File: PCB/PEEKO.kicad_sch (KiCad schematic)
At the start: 26 parts, among them J1 Rasberry PI Pico, J2 Conn_02x15_Odd_Even, J3 Conn_01x02_Pin, J4 Conn_01x02_Pin, U1 TXU0104, U2 TXU0104, U3 TXU0104, U4 TXU0104, U5 TXU0104, U6 TXU0104

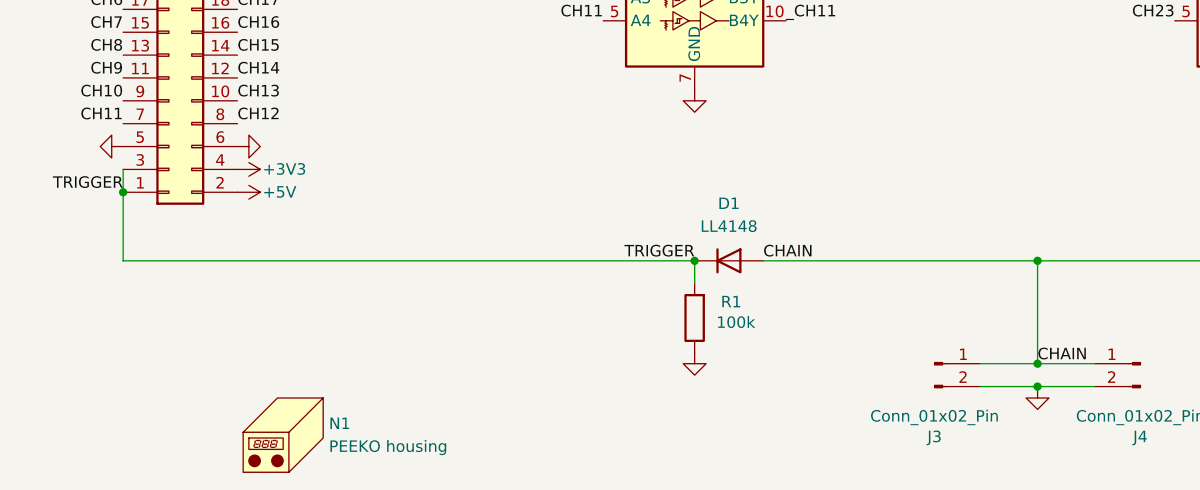
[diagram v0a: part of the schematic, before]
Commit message: boms
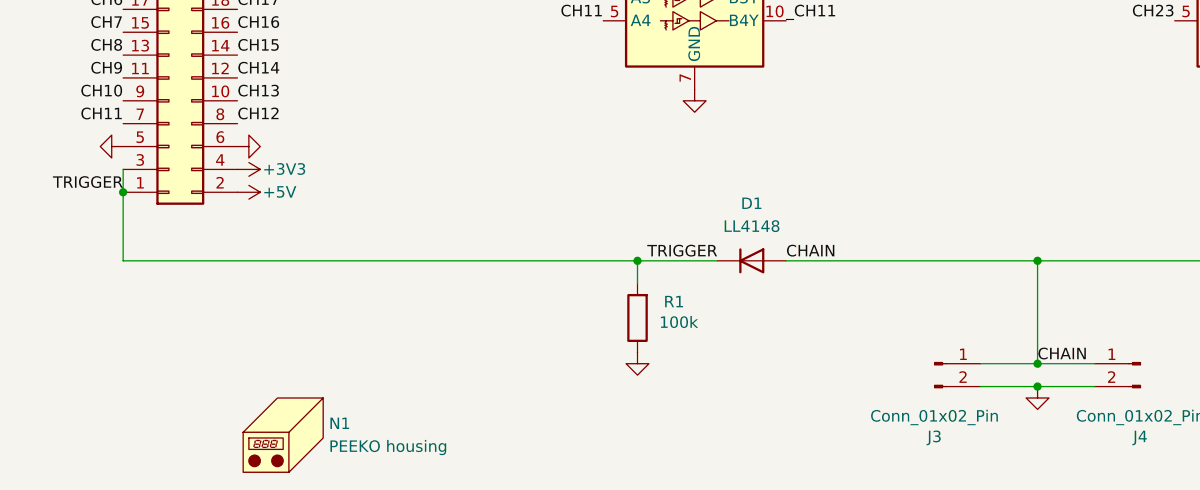
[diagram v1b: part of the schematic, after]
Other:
- moved on the sheet: D1, R1
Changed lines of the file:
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@@
 	)
 	(junction
-		(at 95.25 158.75)
-		(diameter 0)
-		(color 0 0 0 0)
-	)
-	(junction
 		(at 53.34 57.15)
 		(diameter 0)
@@
 	)
 	(junction
+		(at 88.9 158.75)
+		(diameter 0)
+		(color 0 0 0 0)
+	)
+	(junction
 		(at 266.7 101.6)
 		(diameter 0)
@@
 	(wire
 		(pts
-			(xy 95.25 158.75) (xy 95.25 161.29)
+			(xy 223.52 71.12) (xy 223.52 73.66)
 		)
 		(stroke
@@
 	(wire
 		(pts
-			(xy 223.52 71.12) (xy 223.52 73.66)
+			(xy 22.86 41.91) (xy 22.86 44.45)
 		)
 		(stroke
@@
 	(wire
 		(pts
-			(xy 22.86 41.91) (xy 22.86 44.45)
+			(xy 22.86 76.2) (xy 26.67 76.2)
 		)
 		(stroke
@@
 	(wire
 		(pts
-			(xy 22.86 76.2) (xy 26.67 76.2)
+			(xy 22.86 69.85) (xy 22.86 76.2)
 		)
 		(stroke
@@
 	(wire
 		(pts
-			(xy 22.86 69.85) (xy 22.86 76.2)
+			(xy 88.9 158.75) (xy 97.79 158.75)
 		)
 		(stroke
@@
 	(wire
 		(pts
+			(xy 88.9 158.75) (xy 88.9 161.29)
+		)
+		(stroke
+			(width 0)
+			(type default)
+		)
+	)
+	(wire
+		(pts
 			(xy 215.9 121.92) (xy 215.9 114.3)
 		)
@@
 	(wire
 		(pts
-			(xy 102.87 158.75) (xy 133.35 158.75)
+			(xy 105.41 158.75) (xy 133.35 158.75)
 		)
 		(stroke
@@
 	(wire
 		(pts
-			(xy 31.75 158.75) (xy 95.25 158.75)
+			(xy 31.75 158.75) (xy 88.9 158.75)
 		)
 		(stroke
@@
 	)
 	(label "TRIGGER"
-		(at 95.25 158.75 180)
+		(at 97.79 158.75 180)
 		(fields_autoplaced yes)
 		(effects
@@
 	)
 	(label "CHAIN"
-		(at 102.87 158.75 0)
+		(at 105.41 158.75 0)
 		(fields_autoplaced yes)
 		(effects
@@
 	(symbol
 		(lib_id "power:GND")
-		(at 95.25 168.91 0)
+		(at 88.9 168.91 0)
 		(unit 1)
 		(exclude_from_sim no)
@@
 		(fields_autoplaced yes)
 		(property "Reference" "#PWR01"
-			(at 95.25 175.26 0)
+			(at 88.9 175.26 0)
 			(effects
 				(font
@@
 		)
 		(property "Value" "GND"
-			(at 95.25 173.99 0)
+			(at 88.9 173.99 0)
 			(effects
 				(font
@@
 		)
 		(property "Footprint" ""
-			(at 95.25 168.91 0)
+			(at 88.9 168.91 0)
 			(effects
 				(font
@@
 		)
 		(property "Datasheet" ""
-			(at 95.25 168.91 0)
+			(at 88.9 168.91 0)
 			(effects
 				(font
@@
 		)
 		(property "Description" "Power symbol creates a global label with name \"GND\" , ground"
-			(at 95.25 168.91 0)
+			(at 88.9 168.91 0)
 			(effects
 				(font
@@
 	(symbol
 		(lib_id "Device:R")
-		(at 95.25 165.1 180)
+		(at 88.9 165.1 180)
 		(unit 1)
 		(exclude_from_sim no)
@@
 		(dnp no)
 		(property "Reference" "R1"
-			(at 99.314 163.322 0)
+			(at 92.964 163.322 0)
 			(effects
 				(font
@@
 		)
 		(property "Value" "100k"
-			(at 99.822 165.608 0)
+			(at 93.472 165.608 0)
 			(effects
 				(font
@@
 		)
 		(property "Footprint" "000_LOCAL:R_0805"
-			(at 97.028 165.1 90)
+			(at 90.678 165.1 90)
 			(effects
 				(font
@@
 		)
 		(property "Datasheet" "datasheets/PYu-RC_Group_51_RoHS_L_12.pdf"
-			(at 95.25 165.1 0)
+			(at 88.9 165.1 0)
 			(effects
 				(font
@@
 		)
 		(property "Description" "RES 100K OHM 1% 1/8W 0805"
-			(at 95.25 165.1 0)
+			(at 88.9 165.1 0)
 			(effects
 				(font
@@
 		)
 		(property "MPN" "RC0805FR-07100KL"
-			(at 95.25 165.1 0)
+			(at 88.9 165.1 0)
 			(effects
 				(font
@@
 	(symbol
 		(lib_id "000_LOCAL:LL4148")
-		(at 99.06 158.75 0)
+		(at 101.6 158.75 0)
 		(unit 1)
 		(exclude_from_sim no)
@@
 		(fields_autoplaced yes)
 		(property "Reference" "D1"
-			(at 99.06 152.4 0)
+			(at 101.6 152.4 0)
 			(effects
 				(font
@@
 		)
 		(property "Value" "LL4148"
-			(at 99.06 154.94 0)
+			(at 101.6 154.94 0)
 			(effects
 				(font
@@
 		)
 		(property "Footprint" "000_LOCAL:D_MiniMELF"
-			(at 99.06 158.75 0)
+			(at 101.6 158.75 0)
 			(effects
 				(font
@@
 		)
 		(property "Datasheet" "datasheets/ll4148.pdf"
-			(at 99.06 158.75 0)
+			(at 101.6 158.75 0)
 			(effects
 				(font
@@
 		)
 		(property "Description" "50V 1A General Purpose Rectifier Diode"
-			(at 99.06 158.75 0)
+			(at 101.6 158.75 0)
 			(effects
 				(font
@@
 		)
 		(property "MPN" "FDLL4148"
-			(at 99.06 158.75 0)
+			(at 101.6 158.75 0)
 			(effects
 				(font
